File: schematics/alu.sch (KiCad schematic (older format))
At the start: 0 parts

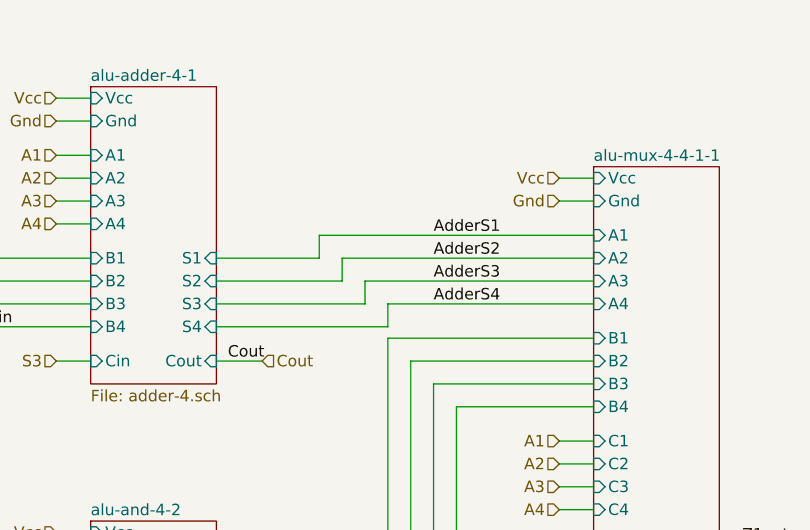
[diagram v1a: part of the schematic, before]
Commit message: ALU appears to work as expected
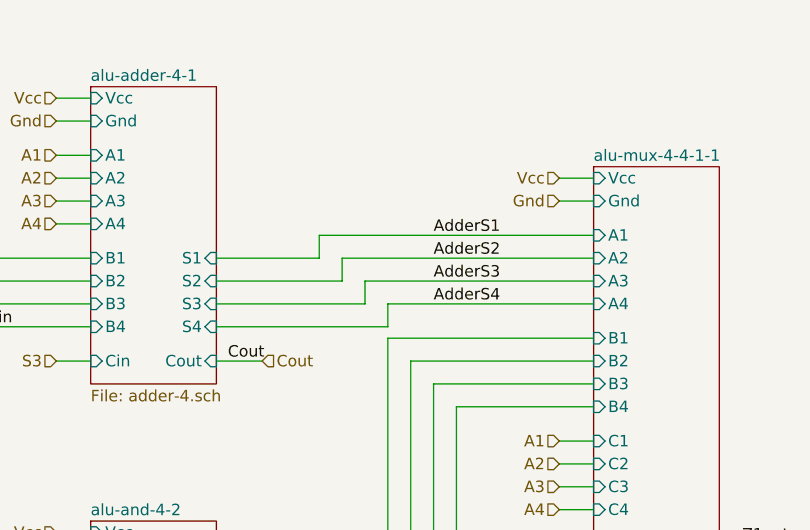
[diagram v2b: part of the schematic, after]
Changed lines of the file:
@@
 Wire Wire Line
 	8550 2250 7900 2250
-Wire Wire Line
-	8450 2150 8450 2050
-Wire Wire Line
-	8450 2050 9550 2050
-Wire Wire Line
-	9550 2050 9550 1950
-Wire Wire Line
-	7900 2150 8450 2150
-Wire Wire Line
-	9550 1950 8350 1950
-Wire Wire Line
-	8350 1950 8350 2050
-Wire Wire Line
-	8350 2050 7900 2050
 Text Label 7950 2500 0    50   ~ 0
 Cout
-Text Label 8850 1950 0    50   ~ 0
-AdderS1
-Text Label 8850 2050 0    50   ~ 0
-AdderS2
 Text Label 8850 2150 0    50   ~ 0
 AdderS3
@@
 Text Label 6650 2350 0    50   ~ 0
 AdderB4in
+Wire Wire Line
+	8450 2150 8450 2050
+Wire Wire Line
+	8450 2050 9550 2050
+Wire Wire Line
+	7900 2150 8450 2150
+Text Label 8850 2050 0    50   ~ 0
+AdderS2
+Text Label 8850 1950 0    50   ~ 0
+AdderS1
+Wire Wire Line
+	7900 2050 8350 2050
+Wire Wire Line
+	8350 2050 8350 1950
+Wire Wire Line
+	8350 1950 9550 1950
 $EndSCHEMATC
